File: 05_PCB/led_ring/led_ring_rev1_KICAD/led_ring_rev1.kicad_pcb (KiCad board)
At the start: 4 copper layers, 24 x 24 mm, 104 parts, among them J1 DATA, J2 POW, U1 74HCT595PW, U2 74HCT595PW, U3 74HCT595PW, U4 74HCT595PW

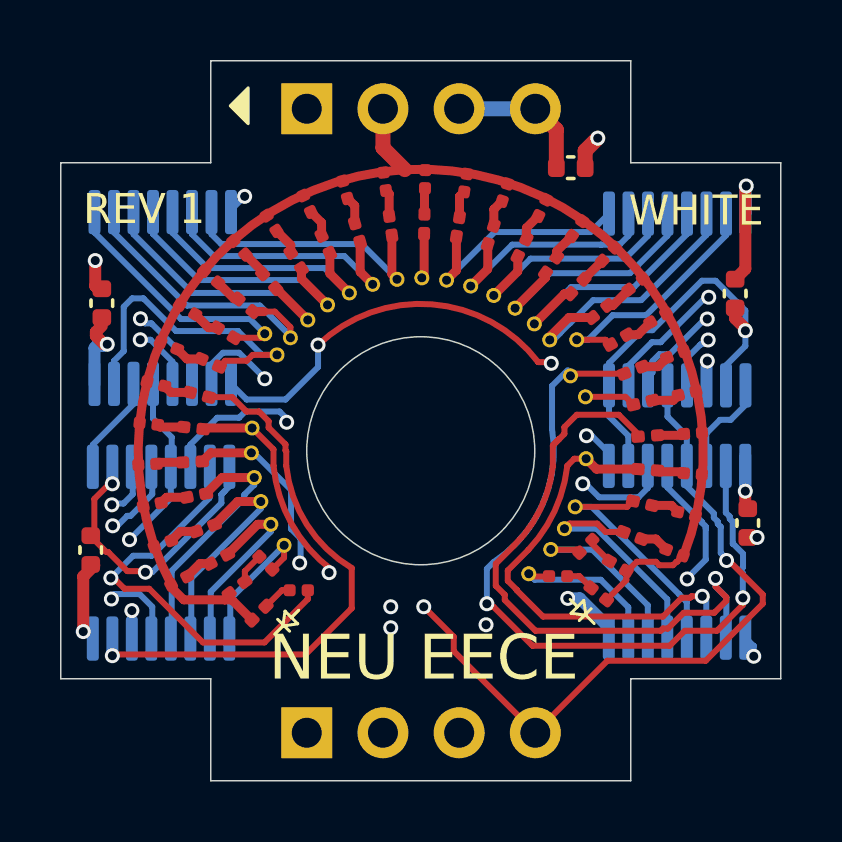
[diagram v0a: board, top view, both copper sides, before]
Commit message: pcbs
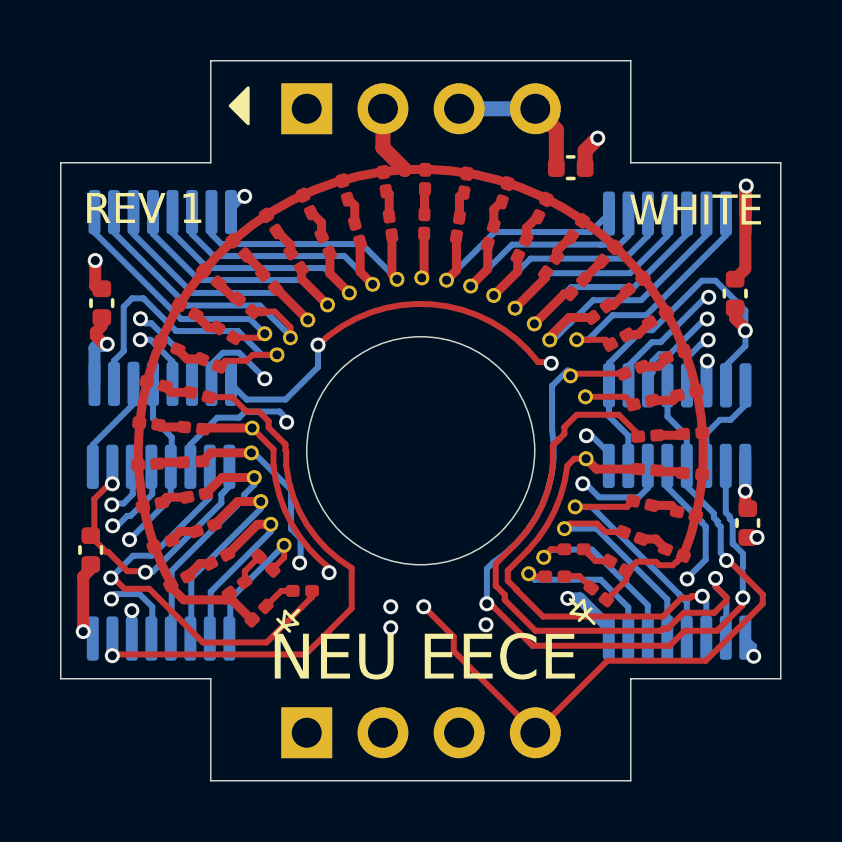
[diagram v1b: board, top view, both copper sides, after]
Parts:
- D1, D10, D11, D12, D13, D14, D15, D16, D17, D18, D19, D2, D20, D21, D22, D23, D24, D25, D26, D27, D28, D29, D3, D30, D31, D32, D4, D5, D6, D7, D8, D9: footprint My Footprints:LED_0201_0603Metric_shift -> My Footprints:LED_0201_0603Metric
- R1, R10, R11, R12, R13, R14, R15, R16, R17, R18, R19, R2, R20, R21, R22, R23, R24, R25, R26, R27, R28, R29, R3, R30, R31, R32, R4, R5, R6, R7, R8, R9: footprint Resistor_SMD:R_0201_0603Metric -> My Footprints:R_0201_0603Metric
- moved R31 0.40 mm to (135.1, 63.3), turned to 180 degrees
- moved V31 0.35 mm to (134.1, 63.6)
- moved R1 0.12 mm to (126.1, 64.7)
- moved R32 0.10 mm to (134.5, 64.2)
